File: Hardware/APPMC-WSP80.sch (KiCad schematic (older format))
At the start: 83 parts, among them J1 + 30V max, J10 STLINK-V3, J101 ADC_C, J102 ADC_D, J14 VDD, J15 PWM, J16 ADC_B, J17 3.0V, J18 1.5V, J2 VOut, J20 ADC_A, J23 GND, J4 Jumper-2B-Open, J6 STLINK-V2, J9 Waveshare 18179, M4 Logo_Open_Hardware_Small, Q1 SI2343CDS-T1-GE3, Q2 ZXMP4A16GTA, Q3 ZXMP4A16GTA, Q4 BSS123, SW1 RESET, U1 INA823, U101 OPA320, U2 3.3V, U3 REF2030, U5 STM32G0B1CEUx, U6 24CW640T-I/OT

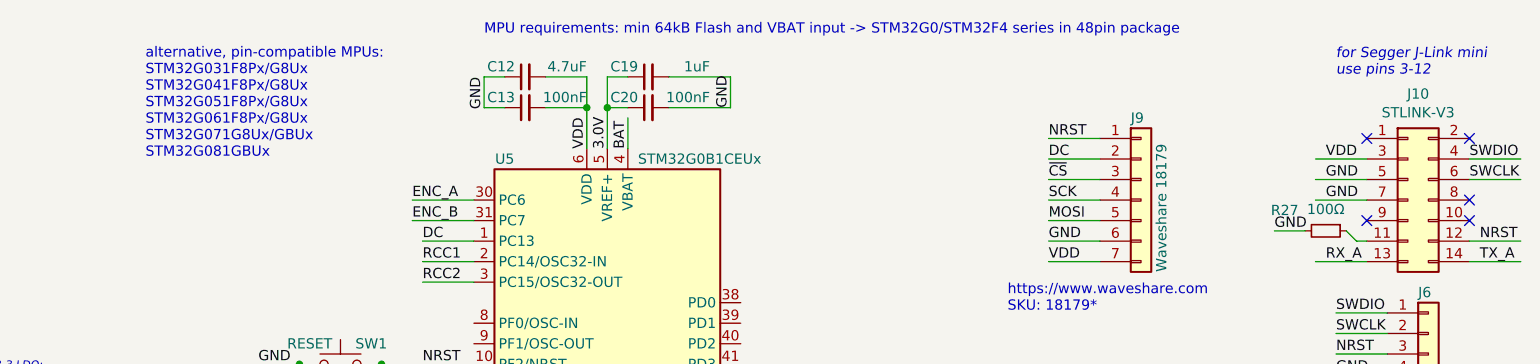
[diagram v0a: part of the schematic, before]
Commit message: MPU list errata
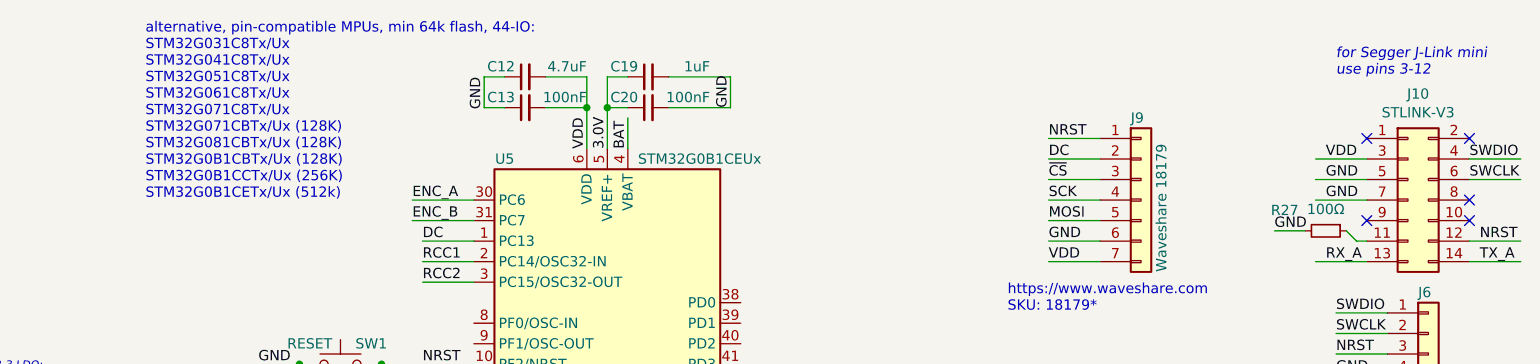
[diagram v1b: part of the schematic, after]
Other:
- note added: "alternative, pin-compatible MPUs, min 64k flash, 44-IO:\nSTM32G031C8Tx/Ux\nSTM32G041C8Tx/Ux\nSTM32G051C8Tx/Ux\nSTM32G061C8Tx/Ux\nSTM32G071C8Tx/Ux\nSTM32G071CBTx/Ux (128K)\nSTM32G081CBTx/Ux (128K)\nSTM32G0B1CBTx/Ux (128K)\nSTM32G0B1CCTx/Ux (256K)\nSTM32G0B1CETx/Ux (512k)"
- note removed: "MPU requirements: min 64kB Flash and VBAT input -> STM32G0/STM32F4 series in 48pin package"
- note removed: "alternative, pin-compatible MPUs:\nSTM32G031F8Px/G8Ux\nSTM32G041F8Px/G8Ux\nSTM32G051F8Px/G8Ux\nSTM32G061F8Px/G8Ux\nSTM32G071G8Ux/GBUx\nSTM32G081GBUx"
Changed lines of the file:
@@
 	0    1    1    0
 $EndComp
-Text Notes 5250 600  0    50   ~ 0
-MPU requirements: min 64kB Flash and VBAT input -> STM32G0/STM32F4 series in 48pin package
 Wire Wire Line
 	4950 1800 5200 1800
@@
 Text Label 4950 2700 0    50   ~ 0
 PWM
-Text Notes 3600 1200 0    50   ~ 0
-alternative, pin-compatible MPUs:\nSTM32G031F8Px/G8Ux\nSTM32G041F8Px/G8Ux\nSTM32G051F8Px/G8Ux\nSTM32G061F8Px/G8Ux\nSTM32G071G8Ux/GBUx\nSTM32G081GBUx
+Text Notes 3600 1400 0    50   ~ 0
+alternative, pin-compatible MPUs, min 64k flash, 44-IO:\nSTM32G031C8Tx/Ux\nSTM32G041C8Tx/Ux\nSTM32G051C8Tx/Ux\nSTM32G061C8Tx/Ux\nSTM32G071C8Tx/Ux\nSTM32G071CBTx/Ux (128K)\nSTM32G081CBTx/Ux (128K)\nSTM32G0B1CBTx/Ux (128K)\nSTM32G0B1CCTx/Ux (256K)\nSTM32G0B1CETx/Ux (512k)
 $Comp
 L STM32G0B1CEUx:STM32G0B1CEUx U5
